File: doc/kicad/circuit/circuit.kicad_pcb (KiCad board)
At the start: 2 copper layers, 49.7 x 53.1 mm, 22 parts, among them J1 4X4 Button Matrix, J1.1 2X2 Matrix A, J1.1.1 Button 1, J1.1.2 Button 2, J1.1.3 Button 5, J1.1.4 Button 6, J1.2 2X2 Matrix B, J1.2.1 Button 3, J1.2.2 Button 4, J1.3 2X2 Matrix C, J1.4 2X2 Matrix D, J3 AVR-ISP, J4 RJ45, SW1 Reset, U1 ATmega328P-P, Y1 Crystal

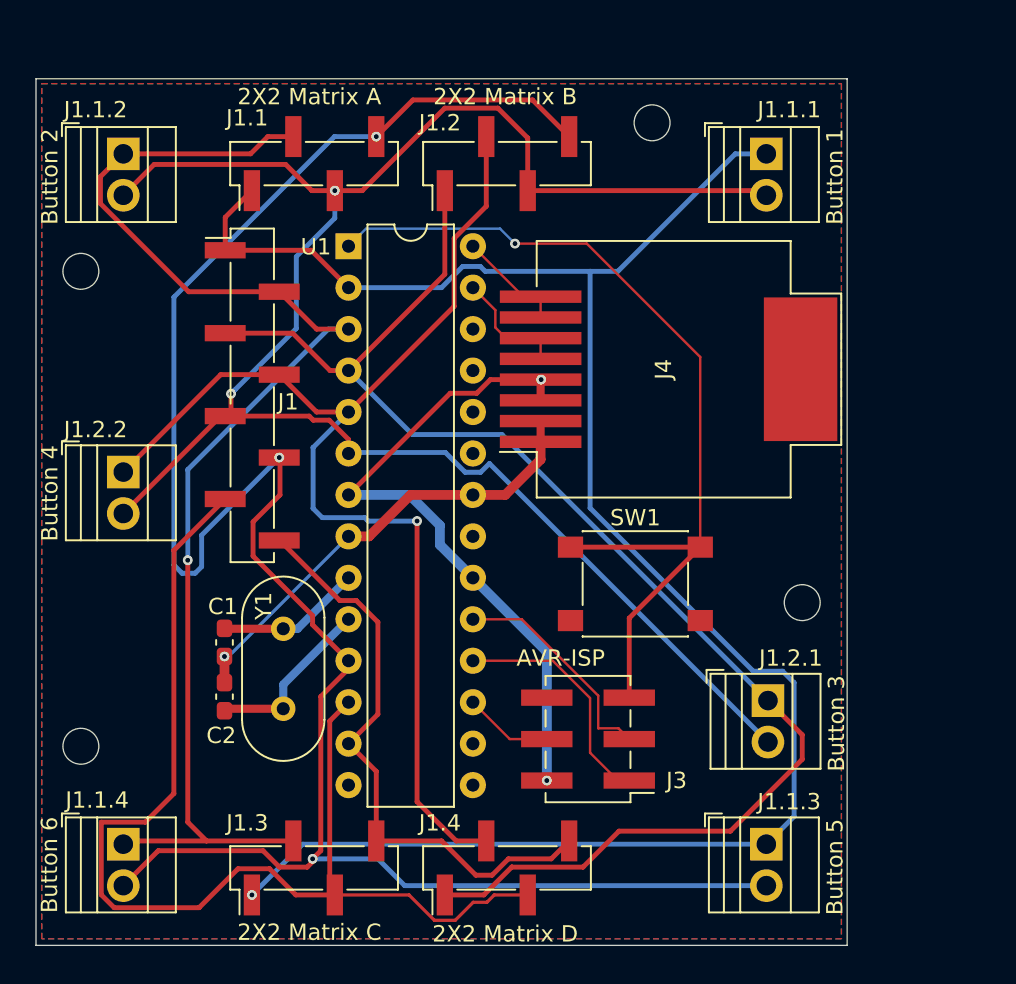
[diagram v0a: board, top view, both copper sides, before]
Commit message: refactor pcb
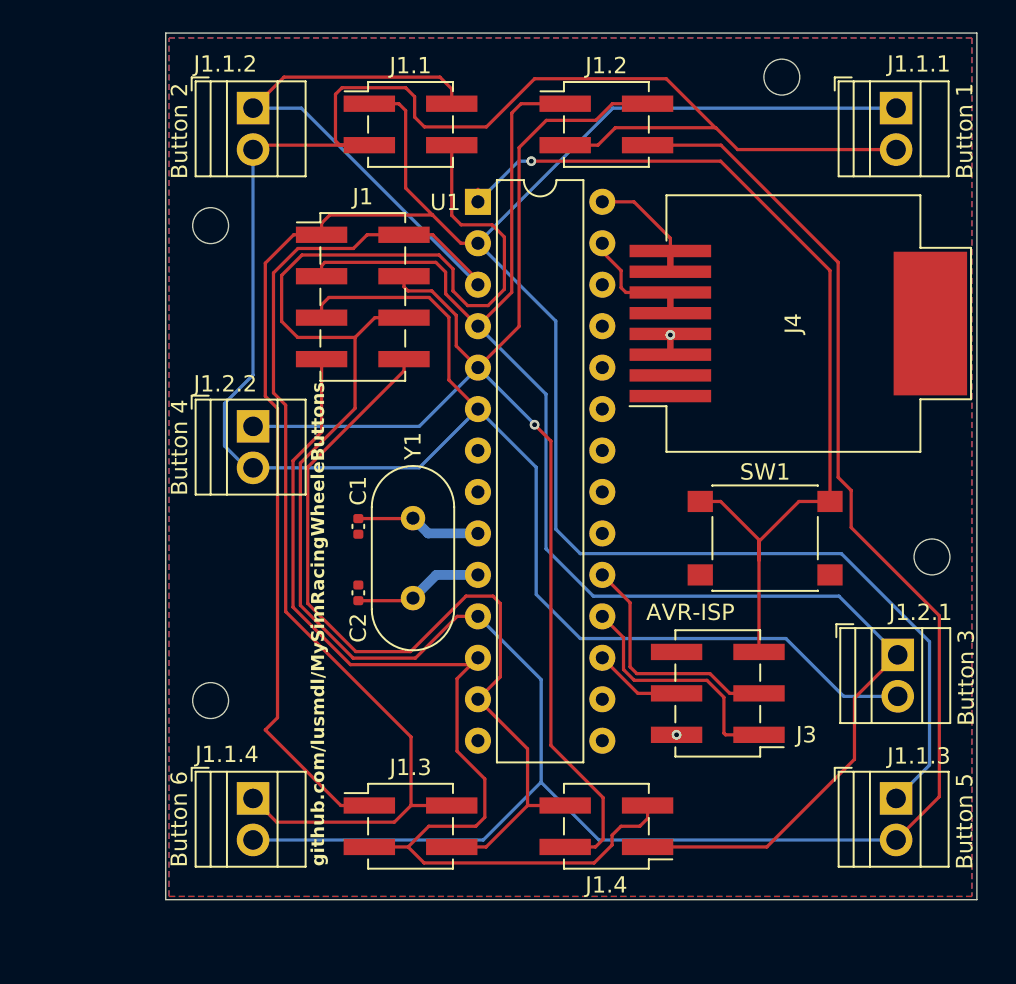
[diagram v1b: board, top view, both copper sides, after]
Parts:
- C1, C2: footprint Capacitor_SMD:C_0603_1608Metric_Pad1.08x0.95mm_HandSolder -> Capacitor_SMD:C_0402_1005Metric
- J1: footprint Connector_PinHeader_2.54mm:PinHeader_1x08_P2.54mm_Vertical_SMD_Pin1Left -> Connector_PinHeader_2.54mm:PinHeader_2x04_P2.54mm_Vertical_SMD
- J1.1: value 2X2 Matrix A -> 2X2 Button Matrix A; footprint Connector_PinHeader_2.54mm:PinHeader_1x04_P2.54mm_Vertical_SMD_Pin1Left -> Connector_PinHeader_2.54mm:PinHeader_2x02_P2.54mm_Vertical_SMD
- J1.2: value 2X2 Matrix B -> 2X2 Button Matrix B; footprint Connector_PinHeader_2.54mm:PinHeader_1x04_P2.54mm_Vertical_SMD_Pin1Left -> Connector_PinHeader_2.54mm:PinHeader_2x02_P2.54mm_Vertical_SMD
- J1.3: value 2X2 Matrix C -> 2X2 Button Matrix C; footprint Connector_PinHeader_2.54mm:PinHeader_1x04_P2.54mm_Vertical_SMD_Pin1Left -> Connector_PinHeader_2.54mm:PinHeader_2x02_P2.54mm_Vertical_SMD
- J1.4: value 2X2 Matrix D -> 2X2 Button Matrix D; footprint Connector_PinHeader_2.54mm:PinHeader_1x04_P2.54mm_Vertical_SMD_Pin1Left -> Connector_PinHeader_2.54mm:PinHeader_2x02_P2.54mm_Vertical_SMD
- moved C1 10.9 mm to (221.8, 72.6)
- moved Y1 10.4 mm to (225.2, 72.1)
- moved C2 10.4 mm to (221.8, 76.7)
- moved J1 9.07 mm to (222.1, 58.6)
- moved SW1 8.43 mm to (246.7, 73.3)
- moved J1.1.1 8.43 mm to (254.8, 47.0)
- moved J1.1.2 8.43 mm to (215.3, 47.0)
- moved J1.1.3 8.43 mm to (254.8, 89.3)
- moved J1.1.4 8.43 mm to (215.3, 89.3)
- moved J1.2.1 8.43 mm to (254.8, 80.5)
- moved J1.2.2 8.43 mm to (215.3, 66.5)
- moved J3 8.43 mm to (243.8, 82.9)
- moved J4 8.43 mm to (248.8, 60.2)
- moved REF** 8.43 mm to (256.9, 74.5)
- moved REF** 8.43 mm to (212.8, 54.2)
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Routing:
- net /R2: track 127.6 -> 178.0 mm, vias 3 -> 0
- net +5V: track 42.0 -> 1.27 mm
- net /R1: track 115.2 -> 151.3 mm, vias 2 -> 0
- net /L1: track 116.9 -> 147.1 mm, vias 1 -> 0
- net GND: track 28.5 -> 0.00 mm, vias 1 -> 0
- net /R4: track 36.5 -> 54.2 mm
- net /L2: track 80.0 -> 96.7 mm, vias 1 -> 0
- net /L4: track 73.5 -> 81.7 mm
- net /L3: track 86.1 -> 92.1 mm
- net /R3: track 70.8 -> 65.1 mm
- net /XTAL2: track 10.8 -> 7.98 mm
- net /XTAL1: track 8.90 -> 7.73 mm
- net /SCK: track 13.8 -> 14.9 mm
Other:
- board text added: "github.com/lusmdl/MySimRacingWheeleButtons"
